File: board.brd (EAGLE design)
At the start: 70 x 70 mm, 6 parts

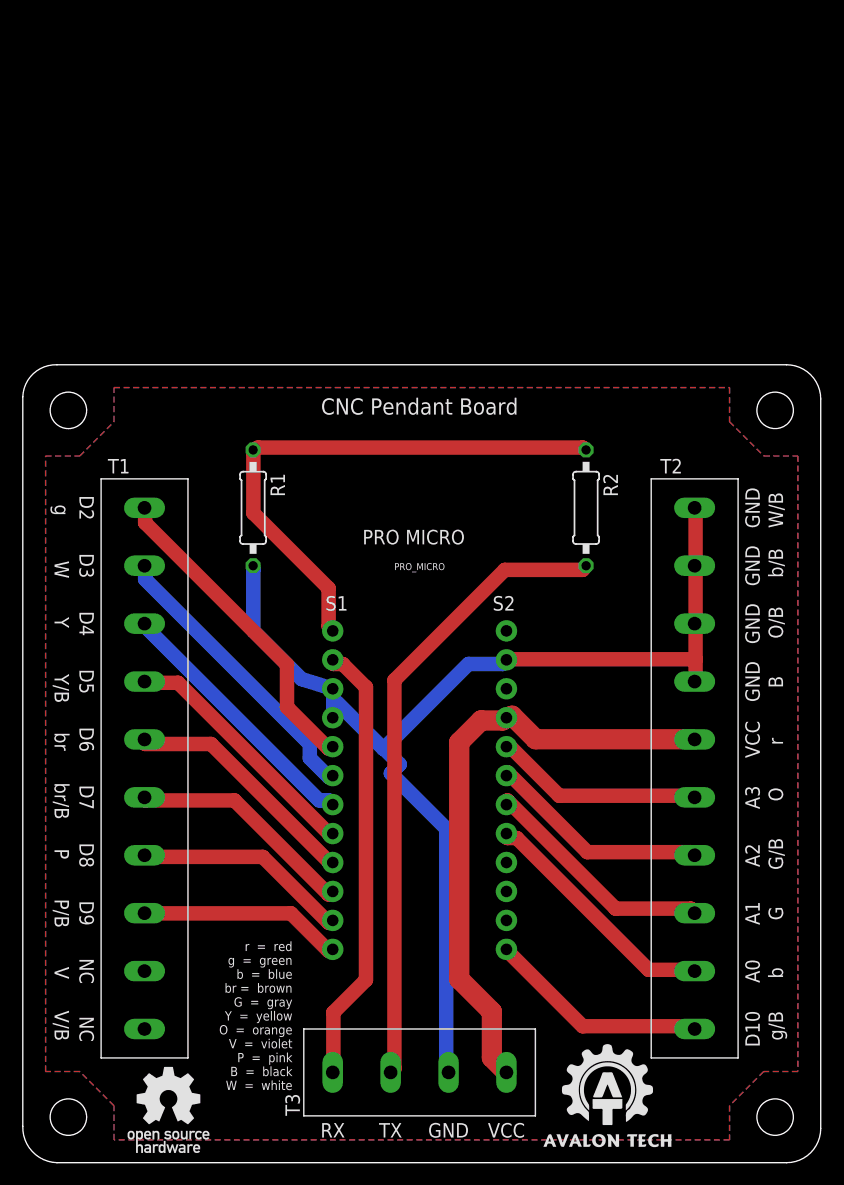
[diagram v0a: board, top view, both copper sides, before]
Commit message: v1.1
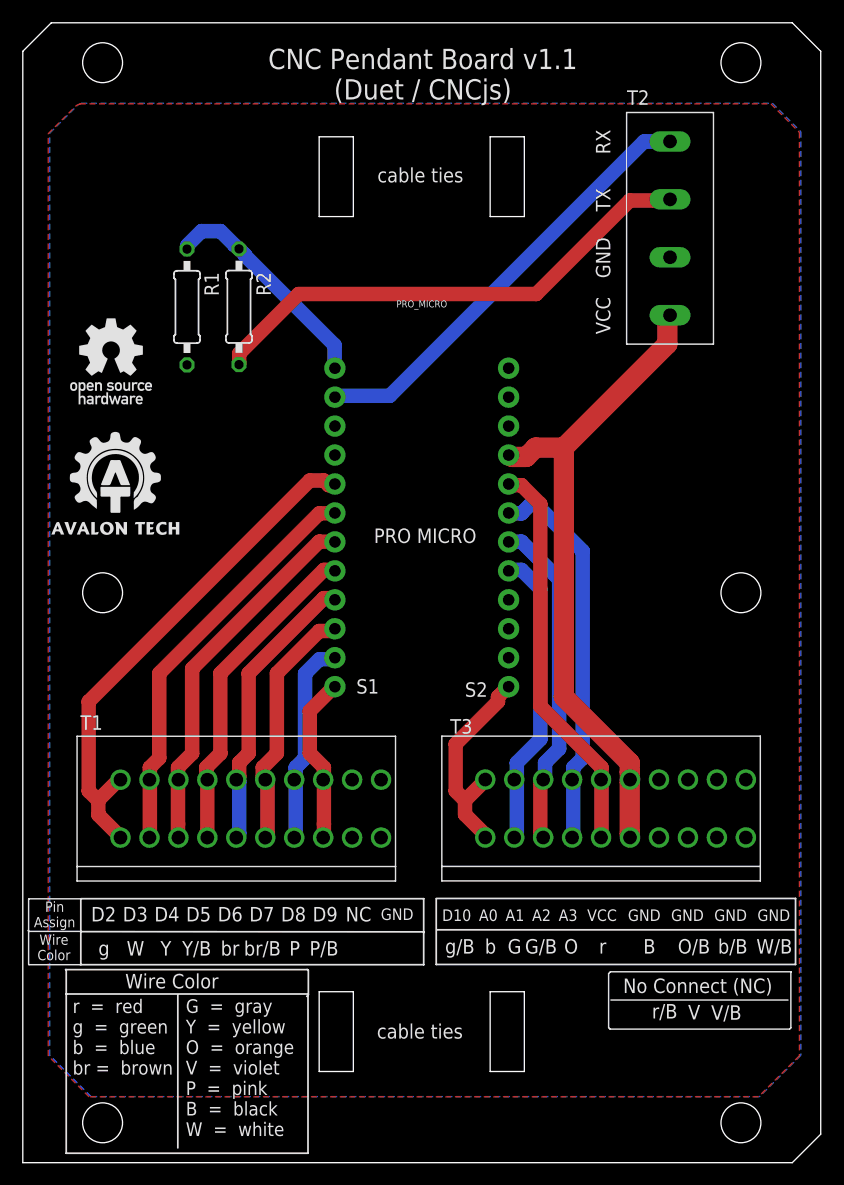
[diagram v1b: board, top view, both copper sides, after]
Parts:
- U$1, U$2: value TERMINAL10 -> KF141V-2.54-10P; device terminals:TERMINAL10 -> terminals:KF141V-2.54-10P
- moved U$3 77.2 mm to (56.8, 82.0), turned to 90 degrees
- moved R2 35.2 mm to (19.0, 75.1)
- moved PRO_MICRO 23.0 mm to (35.0, 57.0)
- moved R1 18.6 mm to (14.4, 75.1)
- moved U$1 9.97 mm to (20.0, 31.1), turned to 180 degrees
- moved U$2 7.78 mm to (52.0, 31.1), turned to 180 degrees
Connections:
- net GND: now also U$1.P$1, U$1.P$2, U$2.P$5, U$2.P$6, U$2.P$7, U$2.P$8
- net N$1: now also U$1.P$19, U$1.P$20; no longer U$1.P$10
- net N$10: now also U$2.P$17, U$2.P$18; no longer U$2.P$9
- net N$11: now also U$2.P$15, U$2.P$16; no longer U$2.P$8
- net N$12: now also U$2.P$13, U$2.P$14; no longer U$2.P$7
- net N$13: now also U$2.P$11, U$2.P$12; no longer U$2.P$6
- net N$2: now also U$1.P$17, U$1.P$18; no longer U$1.P$9
- net N$3: now also U$1.P$15, U$1.P$16; no longer U$1.P$8
- net N$4: now also U$1.P$13, U$1.P$14; no longer U$1.P$7
- net N$5: now also U$1.P$11, U$1.P$12; no longer U$1.P$6
- net N$6: now also U$1.P$10, U$1.P$9; no longer U$1.P$5
- net N$7: now also U$1.P$7, U$1.P$8; no longer U$1.P$4
- net N$8: now also U$1.P$5, U$1.P$6; no longer U$1.P$3
- net N$9: now also U$2.P$19, U$2.P$20; no longer U$2.P$10
- net VCC: now also U$2.P$10, U$2.P$9; no longer U$2.P$5
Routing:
- net GND: track 101.6 -> 0.00 mm
- net N$16: track 48.1 -> 20.0 mm
- net N$1: track 28.2 -> 45.6 mm
- net N$13: track 18.6 -> 35.0 mm
- net N$12: track 19.7 -> 34.1 mm
- net N$18: track 55.5 -> 44.5 mm
- net N$2: track 25.6 -> 36.0 mm
- net N$3: track 23.2 -> 32.5 mm
- net N$11: track 20.9 -> 29.2 mm
- net N$4: track 22.1 -> 28.9 mm
- net N$10: track 21.6 -> 26.4 mm
- net VCC: track 53.1 -> 57.4 mm
- net N$5: track 21.1 -> 25.4 mm
- net N$8: track 17.9 -> 14.7 mm
- net N$6: track 20.2 -> 21.9 mm
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- added copper zone on layer 16, net GND1
- removed copper zone on layer 16, net GND
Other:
- board size 70 x 70 mm -> 70 x 100 mm
- board text added: "CNC Pendant Board v1.1 (Duet / CNCjs)"
- board text added: "G = gray Y = yellow O = orange V = violet P = pink B = black W = white"
- board text added: "No Connect (NC)"
- board text added: "Pin Assign"
- board text added: "Wire Color"
- board text added: "cable ties"
- board text added: "r = red g = green b = blue br = brown"
- board text added: "r/B"
- board text removed: "CNC Pendant Board (Duet / CNCjs)"
- board text removed: "r = red g = green b = blue br = brown G = gray Y = yellow O = orange V = violet P = pink B = black W = white"

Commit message: update
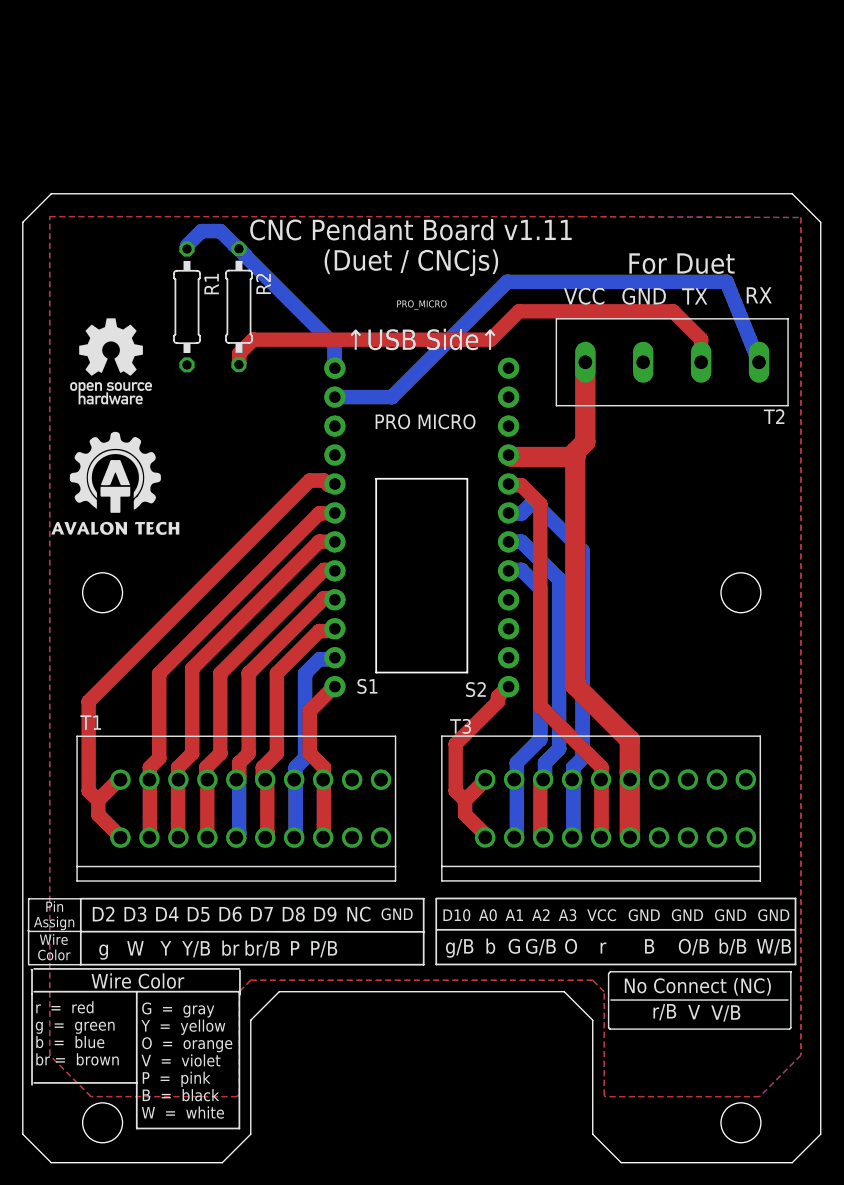
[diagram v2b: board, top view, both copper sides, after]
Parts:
- moved U$3 11.8 mm to (57.0, 70.2), turned to 0 degrees
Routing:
- net N$17: track 38.7 -> 46.2 mm
- net VCC: track 57.4 -> 49.9 mm
- net N$18: track 44.5 -> 46.1 mm
- added copper zone on layer 16, net GND
- removed copper zone on layer 16, net GND1
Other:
- board size 70 x 100 mm -> 70 x 85 mm
- board text added: "CNC Pendant Board v1.11 (Duet / CNCjs)"
- board text added: "For Duet"
- board text added: "↑USB Side↑"
- board text removed: "CNC Pendant Board v1.1 (Duet / CNCjs)"
- board text removed: "cable ties"
